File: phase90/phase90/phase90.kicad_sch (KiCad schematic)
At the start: 46 parts, among them J1 Conn_02x08_Odd_Even, Q1 Q_NJFET_DSG, Q2 Q_NJFET_DSG, Q3 Q_NJFET_DSG, Q4 Q_NJFET_DSG, U10 TL071HIDBVR, U11 TL071HIDBVR, U7 TL071HIDBVR, U8 TL071HIDBVR, U9 TL071HIDBVR

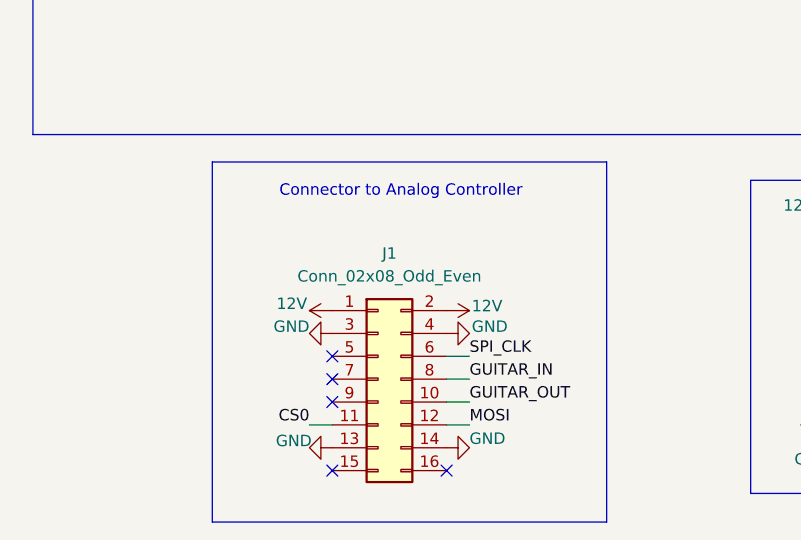
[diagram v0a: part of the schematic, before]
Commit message: fixed connector also?
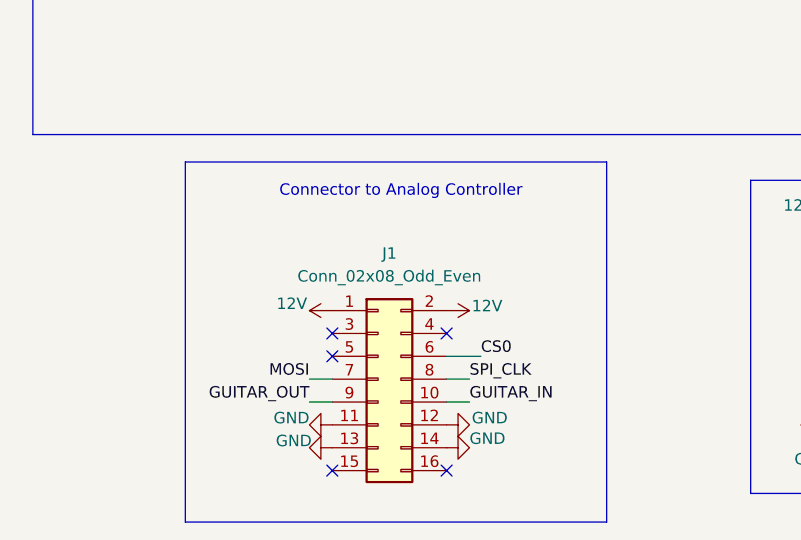
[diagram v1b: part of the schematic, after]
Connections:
- net CS0: now also J1.6 (Pin_6); no longer J1.11 (Pin_11)
- net GND: now also J1.11 (Pin_11), J1.12 (Pin_12); no longer J1.3 (Pin_3), J1.4 (Pin_4)
- net GUITAR_IN: now also J1.10 (Pin_10); no longer J1.8 (Pin_8)
- net GUITAR_OUT: now also J1.9 (Pin_9); no longer J1.10 (Pin_10)
- net MOSI: now also J1.7 (Pin_7); no longer J1.12 (Pin_12)
- net SPI_CLK: now also J1.8 (Pin_8); no longer J1.6 (Pin_6)
